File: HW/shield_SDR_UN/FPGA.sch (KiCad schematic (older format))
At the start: 70 parts, among them J1 Conn_02x09_Odd_Even, J2 Conn_02x08_Odd_Even, U4 XC6SLX9-2TQG144C, X2 ASE-xxxMHz

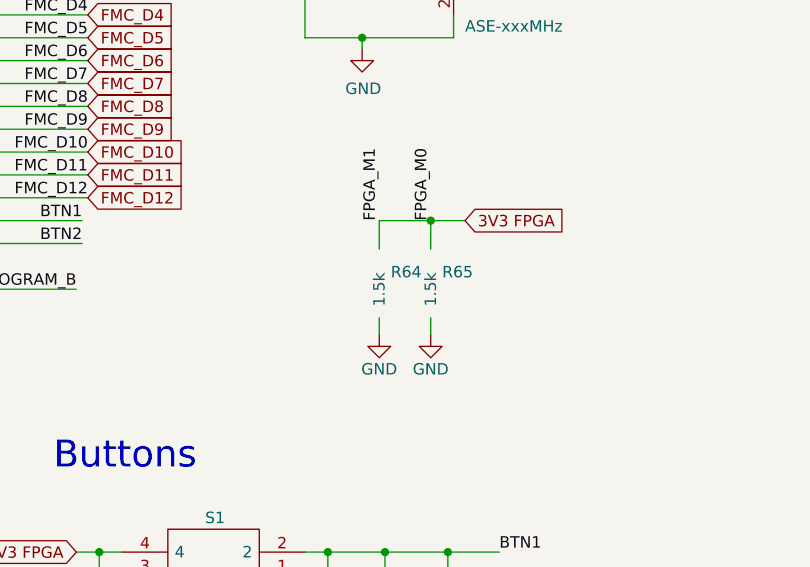
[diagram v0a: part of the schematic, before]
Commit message: PCB_VERSION2
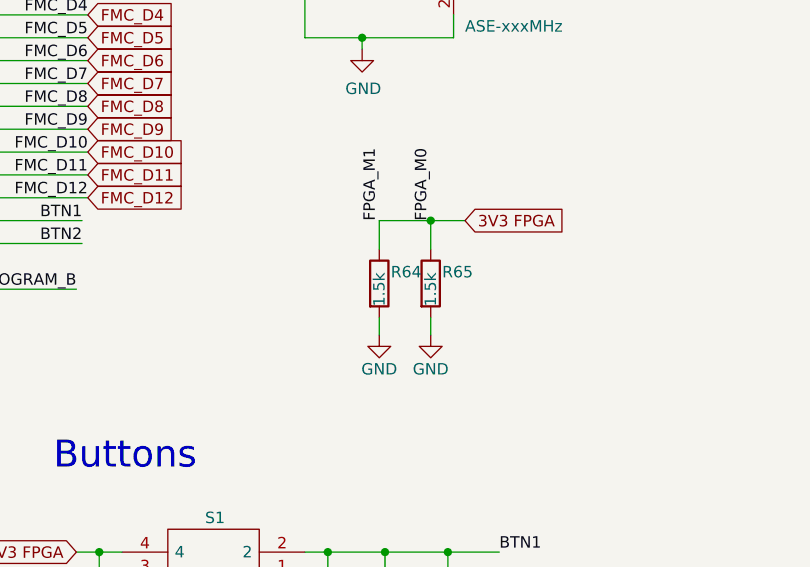
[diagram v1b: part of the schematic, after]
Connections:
- net +3V3: now also R64.1, R65.1
- net GND: now also R64.2, R65.2
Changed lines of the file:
@@
 $Comp
 L Device:R R64
-U 1 0 5CFFF774
+U 1 1 5CFFF774
 P 13975 5775
 F 0 "R64" H 14025 5825 50  0000 L CNN
@@
 $Comp
 L Device:R R65
-U 1 0 5D052DB9
+U 1 1 5D052DB9
 P 14200 5775
 F 0 "R65" H 14250 5825 50  0000 L CNN
